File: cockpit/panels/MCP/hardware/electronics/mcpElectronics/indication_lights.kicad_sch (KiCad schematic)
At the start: 43 parts

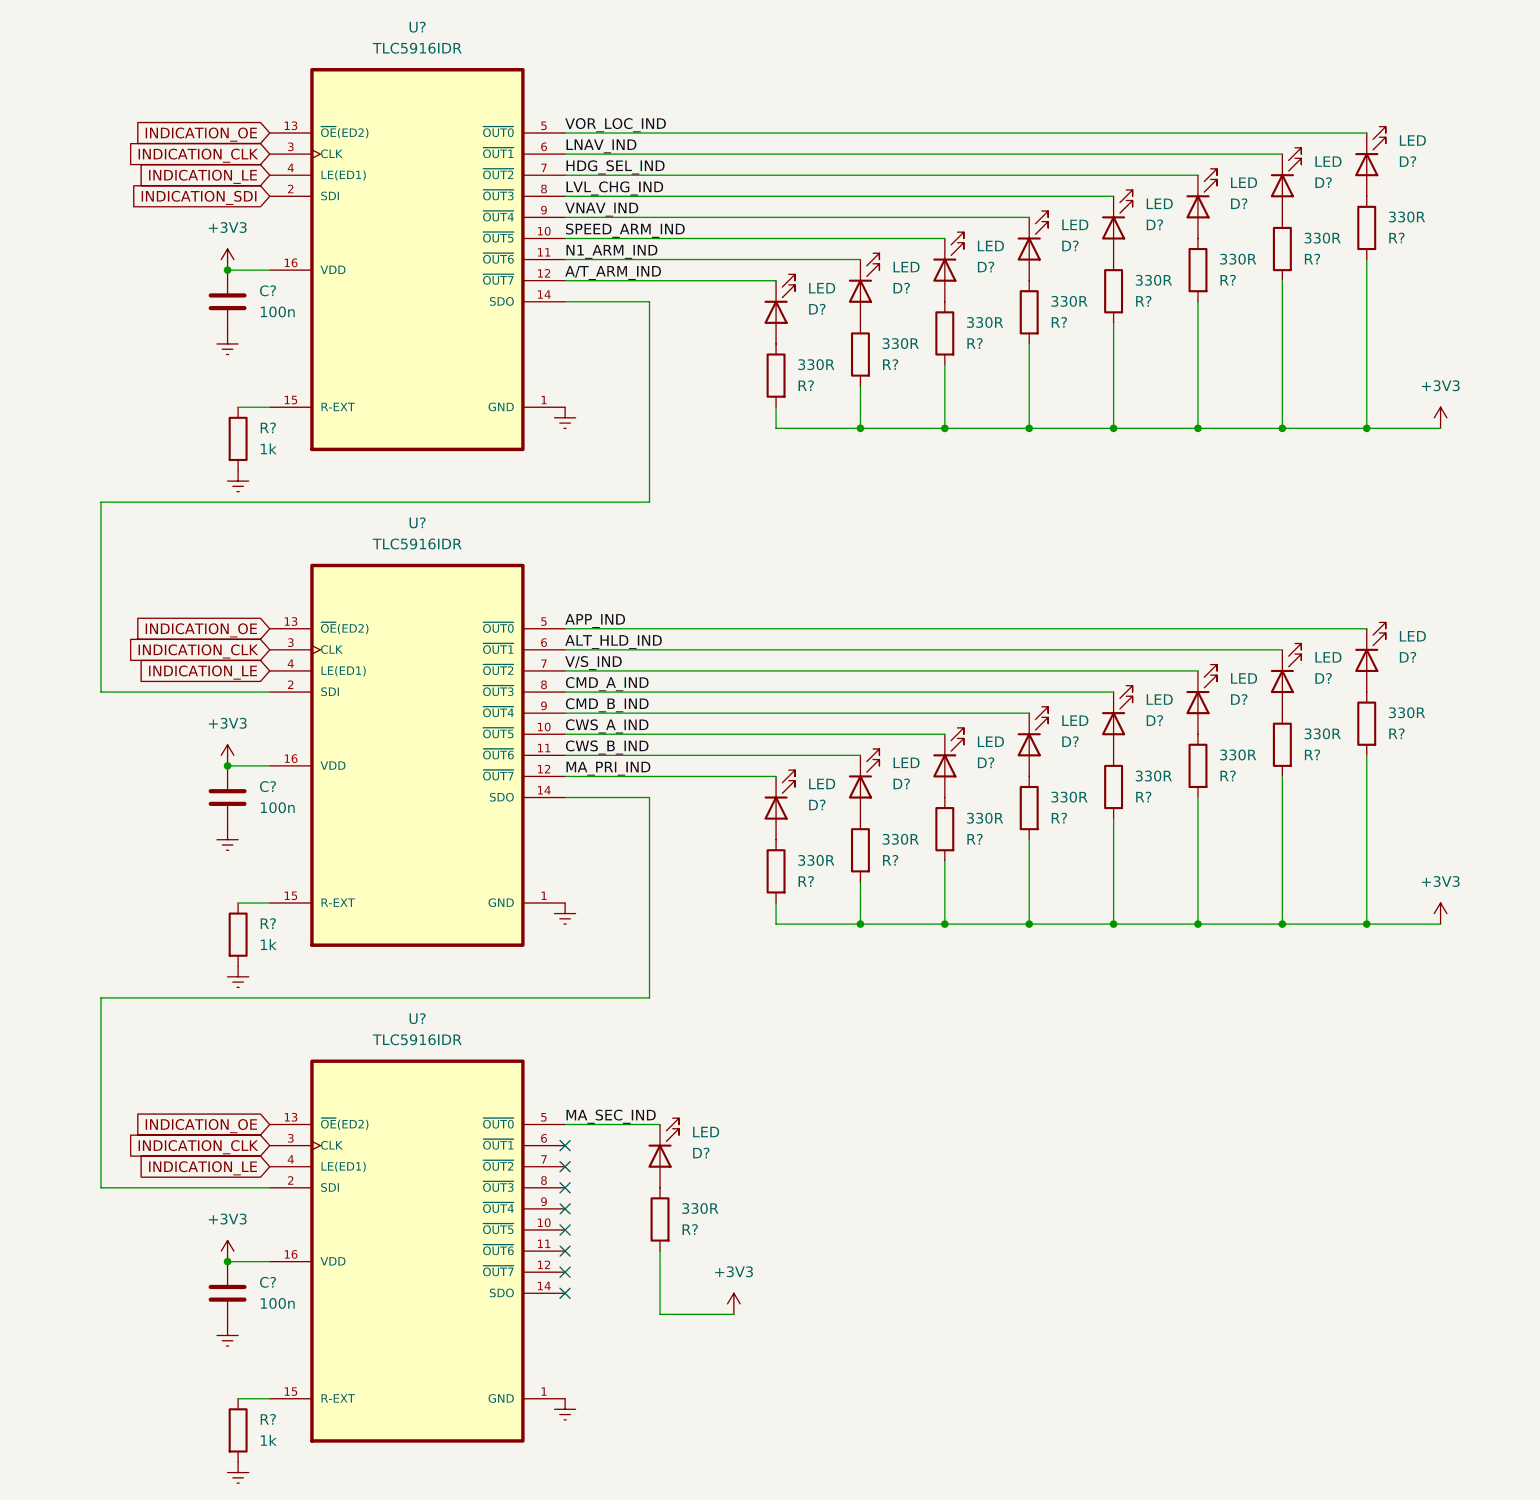
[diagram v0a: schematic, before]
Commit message: update
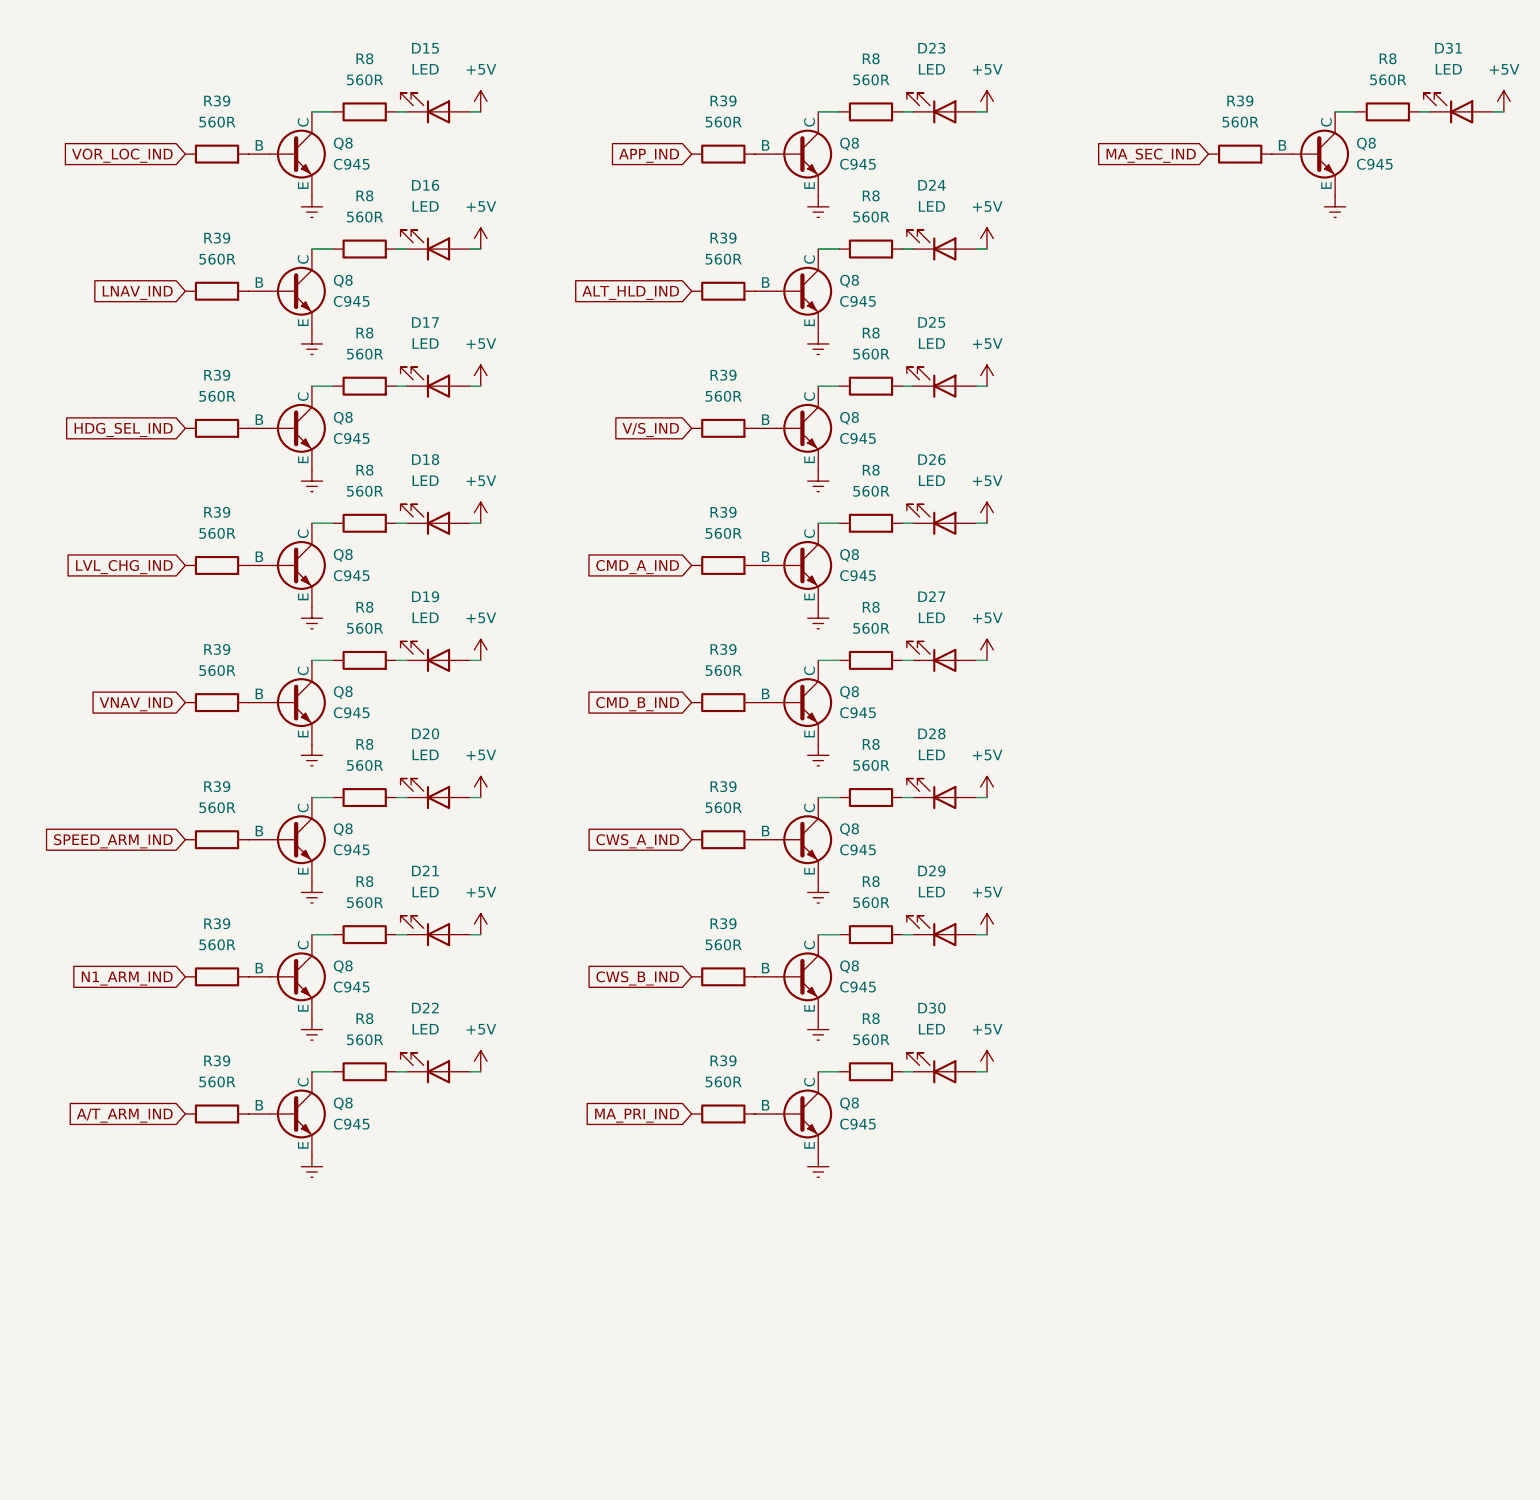
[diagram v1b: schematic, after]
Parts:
- removed C? (x3): 100n, symbol Device:C
- removed D? (x17): LED, symbol Device:LED
- removed R? (x17): 330R, symbol Device:R
- removed R? (x3): 1k, symbol Device:R
- removed U? (x3): TLC5916IDR, TLC5916IDR:SOIC127P600X175-16N, symbol TLC5916IDR:TLC5916IDR
- added D15, D16, D17, D18, D19, D20, D21, D22, D23, D24, D25, D26, D27, D28, D29, D30, D31: LED, Connector_PinHeader_2.54mm:PinHeader_1x02_P2.54mm_Vertical, symbol Device:LED
- added Q8 (x17): C945, Package_TO_SOT_THT:TO-92_Inline, symbol Simulation_SPICE:NPN
- added R39 (x17), R8 (x17): 560R, Resistor_SMD:R_0402_1005Metric, symbol Device:R
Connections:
- net ALT_HLD_IND: now also R39.1
- net APP_IND: now also R39.1
- net A/T_ARM_IND: now also R39.1
- net CMD_A_IND: now also R39.1
- net CMD_B_IND: now also R39.1
- net CWS_A_IND: now also R39.1
- net CWS_B_IND: now also R39.1
- net Earth: now also Q8.3 (E), Q8.3 (E), Q8.3 (E), Q8.3 (E), Q8.3 (E), Q8.3 (E), Q8.3 (E), Q8.3 (E), Q8.3 (E), Q8.3 (E), Q8.3 (E), Q8.3 (E), Q8.3 (E), Q8.3 (E), Q8.3 (E), Q8.3 (E), Q8.3 (E)
- net HDG_SEL_IND: now also R39.1
- net LNAV_IND: now also R39.1
- net LVL_CHG_IND: now also R39.1
- net MA_PRI_IND: now also R39.1
- net MA_SEC_IND: now also R39.1
- net N1_ARM_IND: now also R39.1
- net SPEED_ARM_IND: now also R39.1
- net VNAV_IND: now also R39.1
- net VOR_LOC_IND: now also R39.1
- net V/S_IND: now also R39.1
- new net: D22.1 (K), R8.2
- new net: Q8.1 (C), R8.1 (x17)
- new net: D25.1 (K), R8.2
- new net: D31.1 (K), R8.2
- new net: Q8.2 (B), R39.2 (x17)
- new net: D29.1 (K), R8.2
- new net: D23.1 (K), R8.2
- new net: D27.1 (K), R8.2
- new net: D30.1 (K), R8.2
- new net: D15.1 (K), R8.2
- new net: D21.1 (K), R8.2
- new net: D28.1 (K), R8.2
- new net: D17.1 (K), R8.2
- new net: D18.1 (K), R8.2
- new net: D19.1 (K), R8.2
- new net: D24.1 (K), R8.2
- new net: D26.1 (K), R8.2
- new net: D16.1 (K), R8.2
- new net: D20.1 (K), R8.2
- new net +5V: D15.2 (A), D16.2 (A), D17.2 (A), D18.2 (A), D19.2 (A), D20.2 (A), D21.2 (A), D22.2 (A), D23.2 (A), D24.2 (A), D25.2 (A), D26.2 (A), D27.2 (A), D28.2 (A), D29.2 (A), D30.2 (A), D31.2 (A)
- no-connect marks 8 -> 0
